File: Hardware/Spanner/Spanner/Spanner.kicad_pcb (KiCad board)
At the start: 2 copper layers, 59.8 x 55.2 mm, 69 parts, among them J1 USB_B_Micro, J2 SWD, J3 MOTOR, J4 MOTOR, J5 MOTOR, J6 Conn_01x05_Male, J8 MOTOR, Q1 BC846, Q3 BC846, Q5 BC846, Q6 BC846, U1 STM32L412K8Tx, U2 USBLC6-2SC6, U3 CURRENT_SENS, U4 RFM95W-868S2, U5 MCP1812AT-033/TT, U6 OPA990

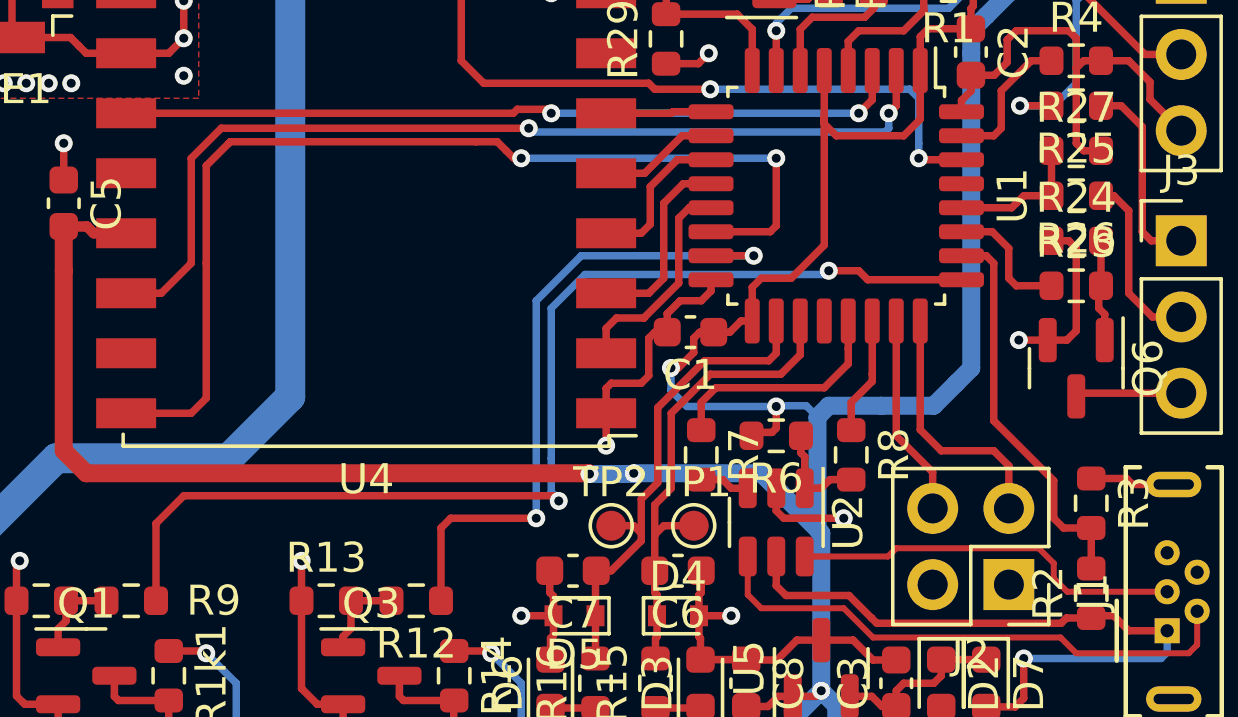
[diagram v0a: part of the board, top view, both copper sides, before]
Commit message: update spanner
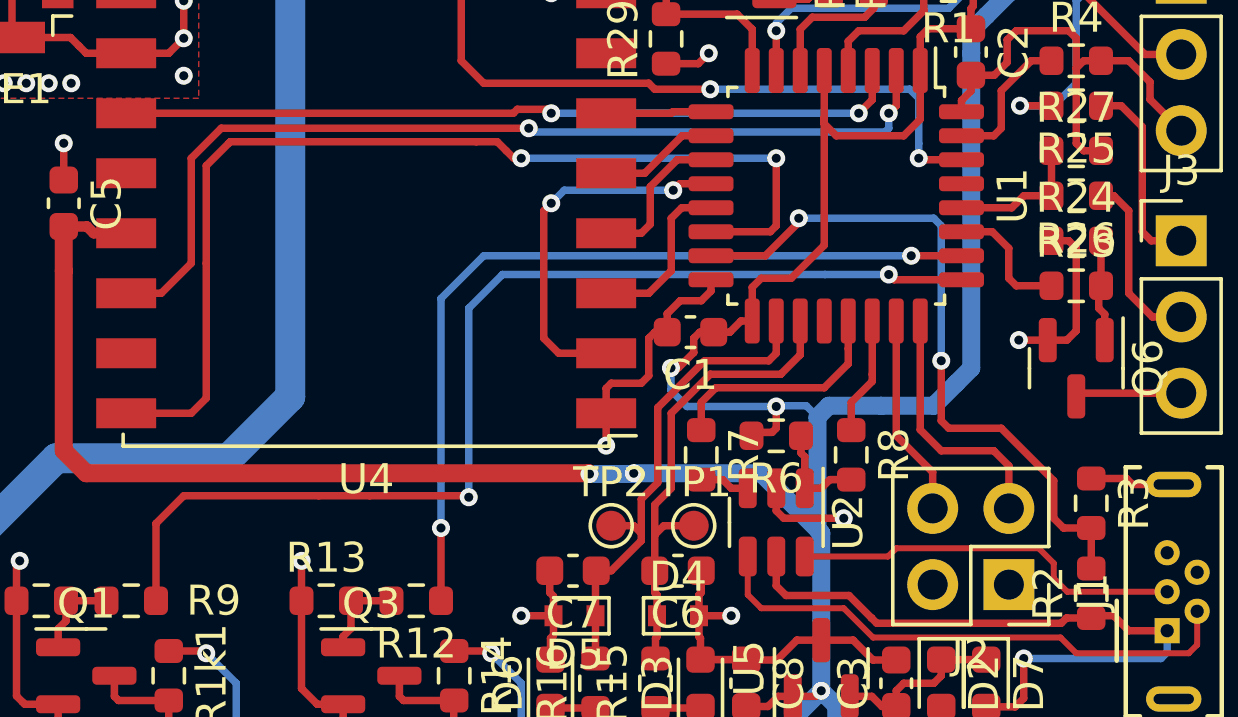
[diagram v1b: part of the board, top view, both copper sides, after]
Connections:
- U1 pad 15: PWM_2 -> VUSB
- U1 pad 26: VUSB -> PWM_2
- U4 pad 2: SPI_MOSI -> SPI_MISO
- U4 pad 3: SPI_MISO -> SPI_MOSI
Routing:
- net VUSB: track 13.2 -> 23.4 mm, vias 0 -> 2
- net SPI_MISO: track 6.47 -> 12.5 mm, vias 0 -> 2
- net PWM_2: track 22.3 -> 28.0 mm
- net SPI_MOSI: track 7.26 -> 5.70 mm
- net PWM_1: track 37.3 -> 36.7 mm
